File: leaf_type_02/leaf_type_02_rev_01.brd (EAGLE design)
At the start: 30 x 16 mm, 21 parts, among them J2 TC_2030_IDC_NL_TOP, J3 CONN_4X1_JST_GH, J6 CONN_4X1_JST_GH, U1 RS485_XCVR_SN65HVD178X

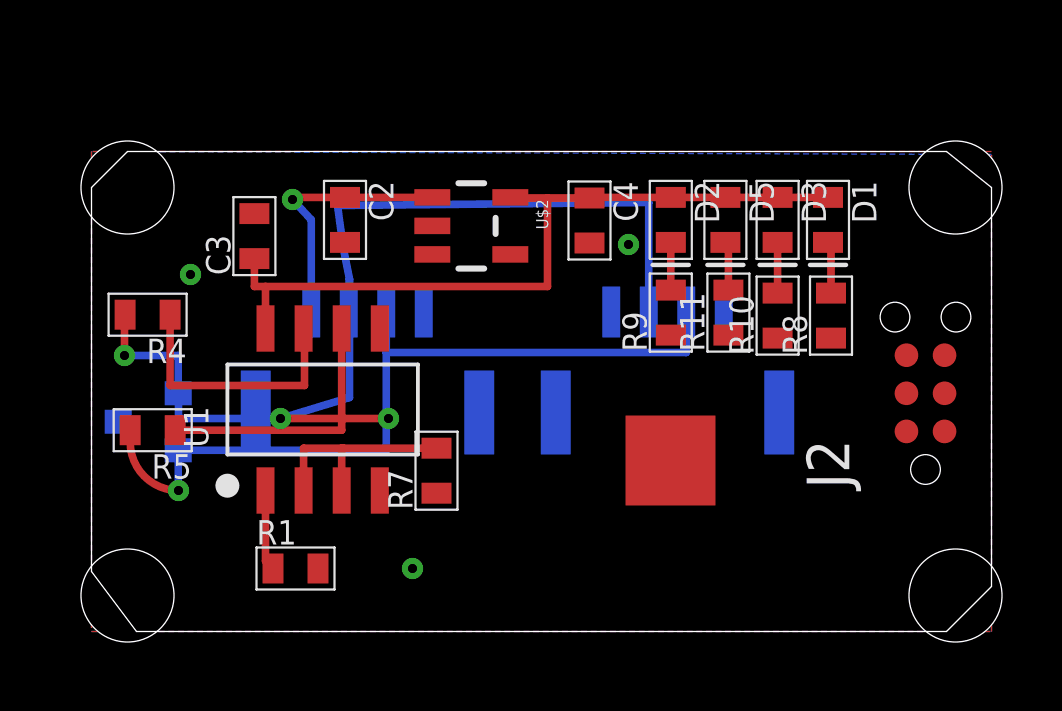
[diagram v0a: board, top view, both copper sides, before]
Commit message: updating 0x02 build
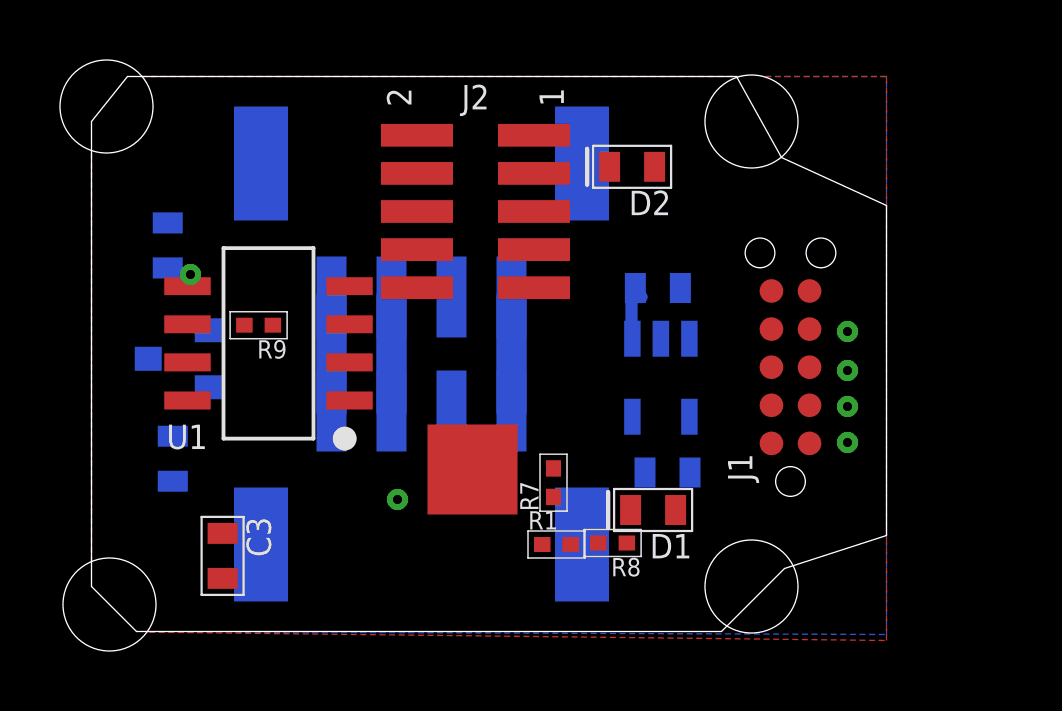
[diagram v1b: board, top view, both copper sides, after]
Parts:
- removed D3, D5: 0603_LED, stepOSP:0603_LED
- removed J3, J6: CONN_4X1_JST_GH, leaf:CONN_4X1_JST_GH
- removed R10, R11: (no value), stepOSP:0603
- added J1: TC_2050_IDC_NL_TOP, leaf:TC_2050_IDC_NL_TOP
- added J4, J5: CONN_4X1_JST_PA, leaf:CONN_4X1_JST_PA
- J2: value TC_2030_IDC_NL_TOP -> CONN_5X2_0P05_IN_SMT; device leaf:TC_2030_IDC_NL_TOP -> leaf:CONN_5X2_0P050_IN_SMT
- R1, R7, R8, R9: device stepOSP:0603 -> stepOSP:0402
- moved J2 17.3 mm to (12.8, 14.0), turned to 270 degrees
- moved R9 13.7 mm to (5.57, 10.2), turned to 180 degrees
- moved D1 11.3 mm to (18.7, 4.05), turned to 180 degrees
- moved C3 10.7 mm to (4.37, 2.52), turned to 270 degrees
- moved C2 10.7 mm to (18.9, 11.4), flipped to the bottom, turned to 180 degrees
- moved R8 10.5 mm to (17.4, 2.95), turned to 180 degrees
- moved C4 8.79 mm to (19.2, 5.30), flipped to the bottom, turned to 180 degrees
- moved R1 8.74 mm to (15.5, 2.90)
- moved U$2 8.10 mm to (19.0, 8.46), flipped to the bottom, turned to 180 degrees
- moved R7 3.92 mm to (15.4, 4.96)
- moved R4 2.41 mm to (2.54, 12.9), flipped to the bottom, turned to 90 degrees
- moved D4 2.33 mm to (2.89, 9.09)
- moved D2 2.19 mm to (18.0, 15.5), turned to 180 degrees
- moved R5 1.16 mm to (2.71, 5.76), flipped to the bottom, turned to 270 degrees
- moved U1 0.32 mm to (5.90, 7.70), turned to 90 degrees
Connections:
- removed net N$4: D3.P$2, R10.P$2
- removed net N$5: D5.P$2, R11.P$2
- net +3V3: no longer D3.P$1, D5.P$1
- net GND1: now also J4.2, J5.3; no longer J3.1, J6.1
- net N$1: now also J4.4, J5.1; no longer J3.3, J6.3
- net N$7: now also J4.3, J5.2; no longer J3.2, J6.2
- net V+: now also J4.1, J5.4; no longer J3.4
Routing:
- net N$1: track 36.2 -> 3.80 mm, vias 3 -> 0
- net +3V3: track 26.5 -> 0.00 mm
- net N$7: track 26.9 -> 3.80 mm, vias 1 -> 0
- net N$9: track 8.94 -> 0.00 mm
- net N$6: track 8.77 -> 0.00 mm
- net N$10: track 7.25 -> 0.00 mm
- net V+: track 8.68 -> 5.91 mm, vias 1 -> 0
- net N$12: track 2.70 -> 0.00 mm
- net N$2: track 1.73 -> 0.00 mm
- net N$4: track 1.69 -> 0.00 mm
- net N$5: track 1.63 -> 0.00 mm
- net N$3: track 1.59 -> 0.00 mm
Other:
- board size 30 x 16 mm -> 26.5 x 18.5 mm
